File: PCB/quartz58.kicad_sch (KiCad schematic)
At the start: 194 parts, among them J1 OLED_128x32, J2 OLED_128x32, J3 Conn_01x10_Socket, J4 Conn_01x10_Pin, SW1 SW_SPDT, SW2 SW_Push, SW3 SW_SPDT, SW4 SW_Push, T1 TPS65-201A-S, U1 Nice_Nano_V2, U2 Nice_Nano_V2

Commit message: updates to pcb
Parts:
- T1: footprint (none) -> Connector_FFC-FPC:Hirose_FH12-6S-0.5SH_1x06-1MP_P0.50mm_Horizontal
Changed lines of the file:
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@@
 			)
 		)
-		(property "Footprint" ""
+		(property "Footprint" "Connector_FFC-FPC:Hirose_FH12-6S-0.5SH_1x06-1MP_P0.50mm_Horizontal"
 			(at 288.29 185.42 0)
 			(effects

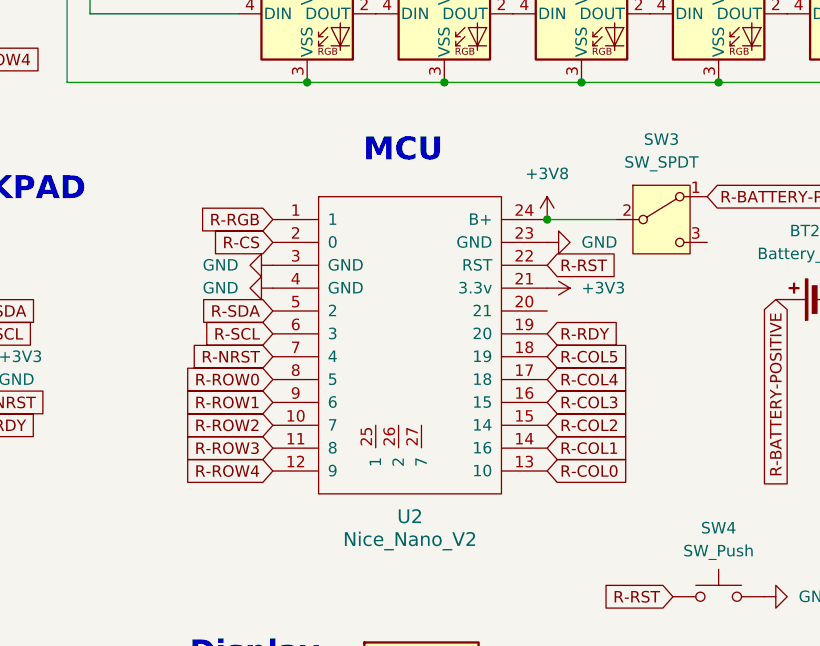
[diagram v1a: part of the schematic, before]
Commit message: more progress
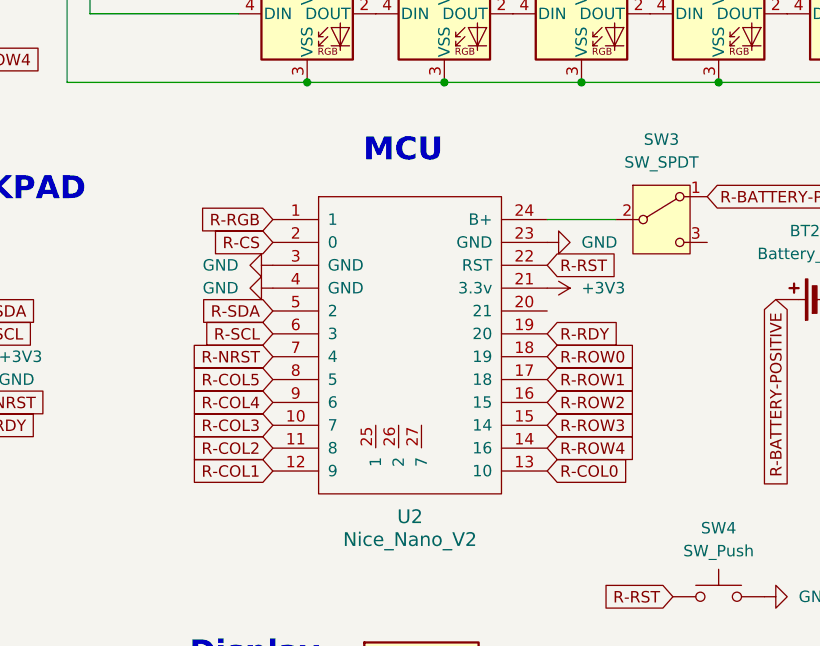
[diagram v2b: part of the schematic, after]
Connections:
- net R-COL1: now also U2.12 (9); no longer U2.14 (16)
- net R-COL2: now also U2.11 (8); no longer U2.15 (14)
- net R-COL3: now also U2.10 (7); no longer U2.16 (15)
- net R-COL4: now also U2.9 (6); no longer U2.17 (18)
- net R-COL5: now also U2.8 (5); no longer U2.18 (19)
- net R-ROW0: now also U2.18 (19); no longer U2.8 (5)
- net R-ROW1: now also U2.17 (18); no longer U2.9 (6)
- net R-ROW2: now also U2.16 (15); no longer U2.10 (7)
- net R-ROW3: now also U2.15 (14); no longer U2.11 (8)
- net R-ROW4: now also U2.14 (16); no longer U2.12 (9)
- net +3V8: no longer names the net of SW3.2 (B), U2.24 (B+)

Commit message: updates
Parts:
- BT1, BT2: footprint ScottoKeebs_Components:Connector_1x02_JST-PH -> Connector_JST:JST_PH_S2B-PH-K_1x02_P2.00mm_Horizontal
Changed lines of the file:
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@@
 			)
 		)
-		(property "Footprint" "ScottoKeebs_Components:Connector_1x02_JST-PH"
+		(property "Footprint" "Connector_JST:JST_PH_S2B-PH-K_1x02_P2.00mm_Horizontal"
 			(at 101.346 173.99 90)
 			(effects
@@
 			)
 		)
-		(property "Footprint" "ScottoKeebs_Components:Connector_1x02_JST-PH"
+		(property "Footprint" "Connector_JST:JST_PH_S2B-PH-K_1x02_P2.00mm_Horizontal"
 			(at 388.366 177.8 90)
 			(effects
